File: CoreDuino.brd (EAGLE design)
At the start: 25 x 25 mm, 18 parts, among them U1 ATMEGA328P_TQFP

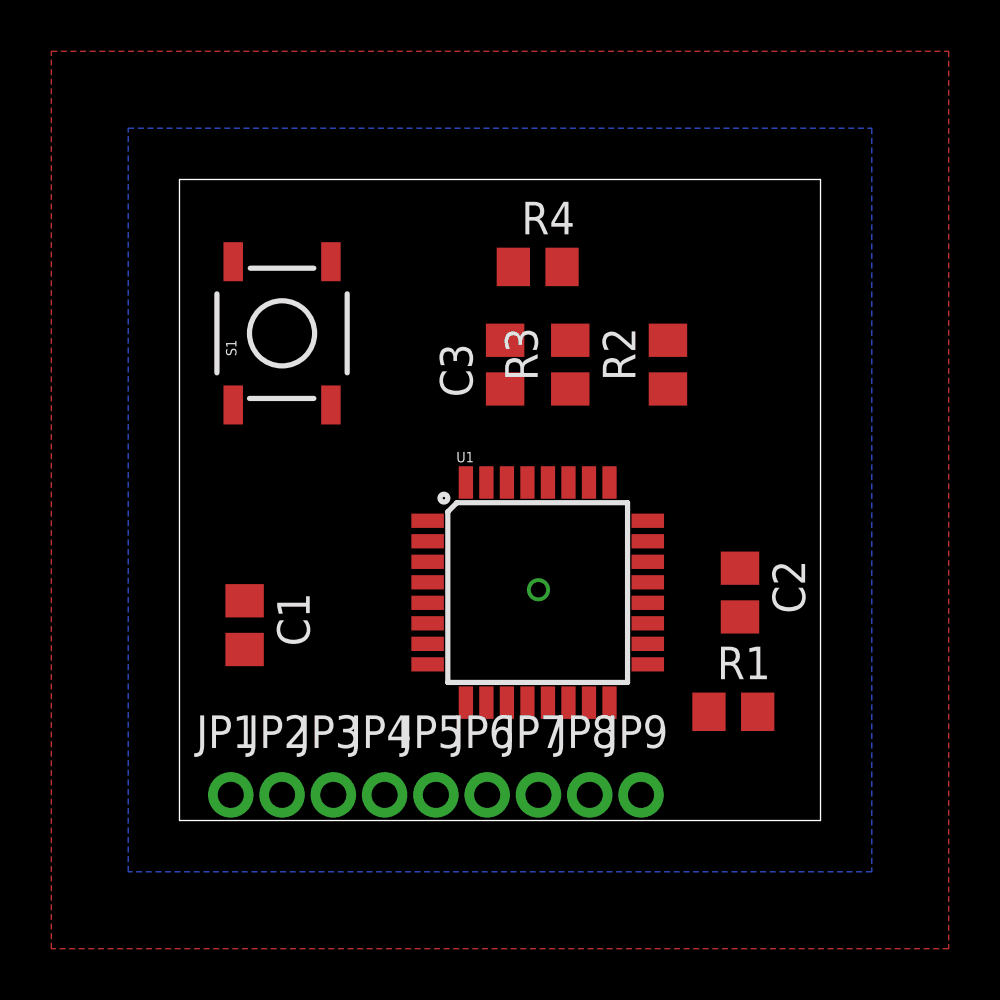
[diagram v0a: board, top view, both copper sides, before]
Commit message: More Changes
More Changes
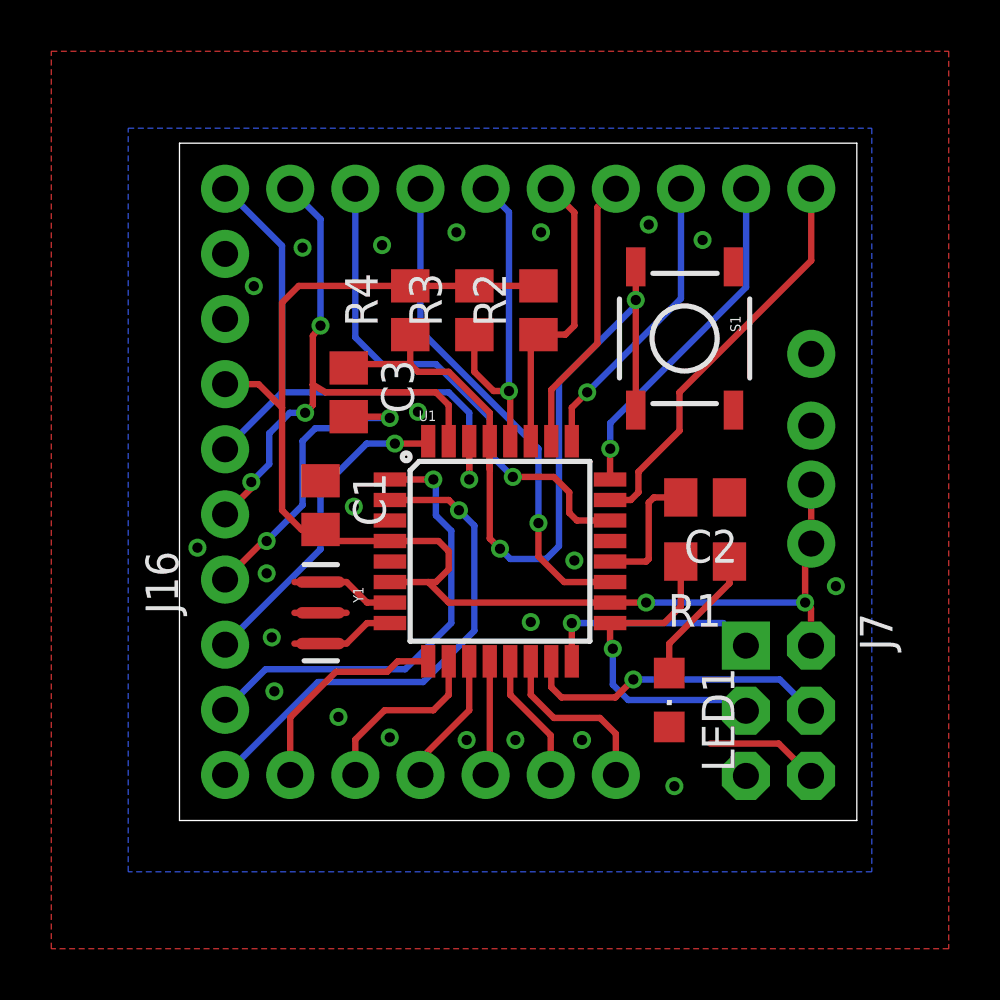
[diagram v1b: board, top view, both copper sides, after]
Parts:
- removed JP1, JP2, JP3, JP4, JP5, JP6, JP7, JP8, JP9: (no value), adafruit:1X01-CLEANBIG
- added J1, J10, J11, J12, J13, J14, J15, J17, J18, J19, J2, J20, J21, J22, J23, J24, J25, J3, J4, J5, J6, J8, J9: (no value), SparkFun-Connectors:1X01NS-KIT
- added J16: (no value), SparkFun-Connectors:1X06_NO_SILK
- added J7: AVR_SPI_PRG_6NS, SparkFun-Connectors:2X3-NS
- added LED1: (no value), adafruit:CHIPLED_0805
- added Y1: 16MHZ, SparkFun-FreqCtrl:RESONATOR-SMD
- moved S1 15.7 mm to (19.7, 18.8), turned to 270 degrees
- moved C3 6.19 mm to (6.60, 16.7), turned to 270 degrees
- moved R1 5.96 mm to (20.5, 10.1), turned to 180 degrees
- moved C1 5.54 mm to (5.50, 12.3)
- moved R2 5.48 mm to (14.0, 19.9)
- moved R4 5.25 mm to (9.00, 19.9), turned to 90 degrees
- moved R3 4.30 mm to (11.5, 19.9)
- moved C2 3.95 mm to (20.5, 12.6), turned to 180 degrees
- moved U1 2.18 mm to (12.5, 10.5)
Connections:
- net N$2 renamed RESET
- removed net N$4: R2.1, U1.27
- removed net N$5: R3.1, U1.28
- new net A0: J1.1, U1.23
- new net A1: J2.1, U1.24
- new net A2: J3.1, U1.25
- new net A3: J17.1, U1.26
- new net A4: J20.1, R2.1, U1.27
- new net A5: J21.1, R3.1, U1.28
- new net A6: J18.1, U1.19
- new net A7: J19.1, U1.22
- new net D10: J6.1, U1.14
- new net D2: J11.1, U1.32
- new net D3: J12.1, U1.1
- new net D4: J13.1, U1.2
- new net D5: J14.1, U1.9
- new net D6: J15.1, U1.10
- new net D7: J8.1, U1.11
- new net D8: J4.1, U1.12
- new net D9: J5.1, U1.13
- new net DTR: C3.2, J16.1
- new net MISO: J7.1, U1.16
- new net MOSI: J7.4, U1.15
- new net N$2: U1.8, Y1.3
- new net RST: J7.5
- new net RXI: J16.3, J9.1, U1.30
- new net SCK: J7.3, R1.2, U1.17
- new net TXO: J10.1, J16.2, U1.31
- net GND: now also J16.5, J16.6, J24.1, J25.1, J7.6, LED1.C, Y1.2
- net N$1: now also LED1.A, R1.1; no longer C3.2
- net N$6: now also U1.7, Y1.1; no longer R1.2, U1.17
- net VCC: now also J16.4, J22.1, J23.1, J7.2
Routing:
- net VCC: track 0.00 -> 52.8 mm, vias 0 -> 2
- net RESET: track 0.00 -> 33.5 mm, vias 0 -> 2
- net RXI: track 0.00 -> 23.7 mm, vias 0 -> 1
- net TXO: track 0.00 -> 22.1 mm, vias 0 -> 3
- net A7: track 0.00 -> 20.0 mm, vias 0 -> 1
- net D4: track 0.00 -> 19.9 mm, vias 0 -> 1
- net A6: track 0.00 -> 19.5 mm, vias 0 -> 1
- net D3: track 0.00 -> 17.8 mm, vias 0 -> 1
- net A0: track 0.00 -> 15.9 mm
- net A1: track 0.00 -> 13.5 mm, vias 0 -> 1
- net A5: track 0.00 -> 13.4 mm, vias 0 -> 1
- net SCK: track 0.00 -> 12.8 mm, vias 0 -> 1
- net D2: track 0.00 -> 12.6 mm, vias 0 -> 1
- net DTR: track 0.00 -> 12.1 mm, vias 0 -> 2
- net MOSI: track 0.00 -> 12.1 mm, vias 0 -> 1
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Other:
- board size 25 x 25 mm -> 26.4 x 26.4 mm
